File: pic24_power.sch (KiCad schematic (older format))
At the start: 12 parts, among them P2 BAT_CONN, P3 PWR_SWITCH, U1 PIC24EP256GP204, U3 TLV1117

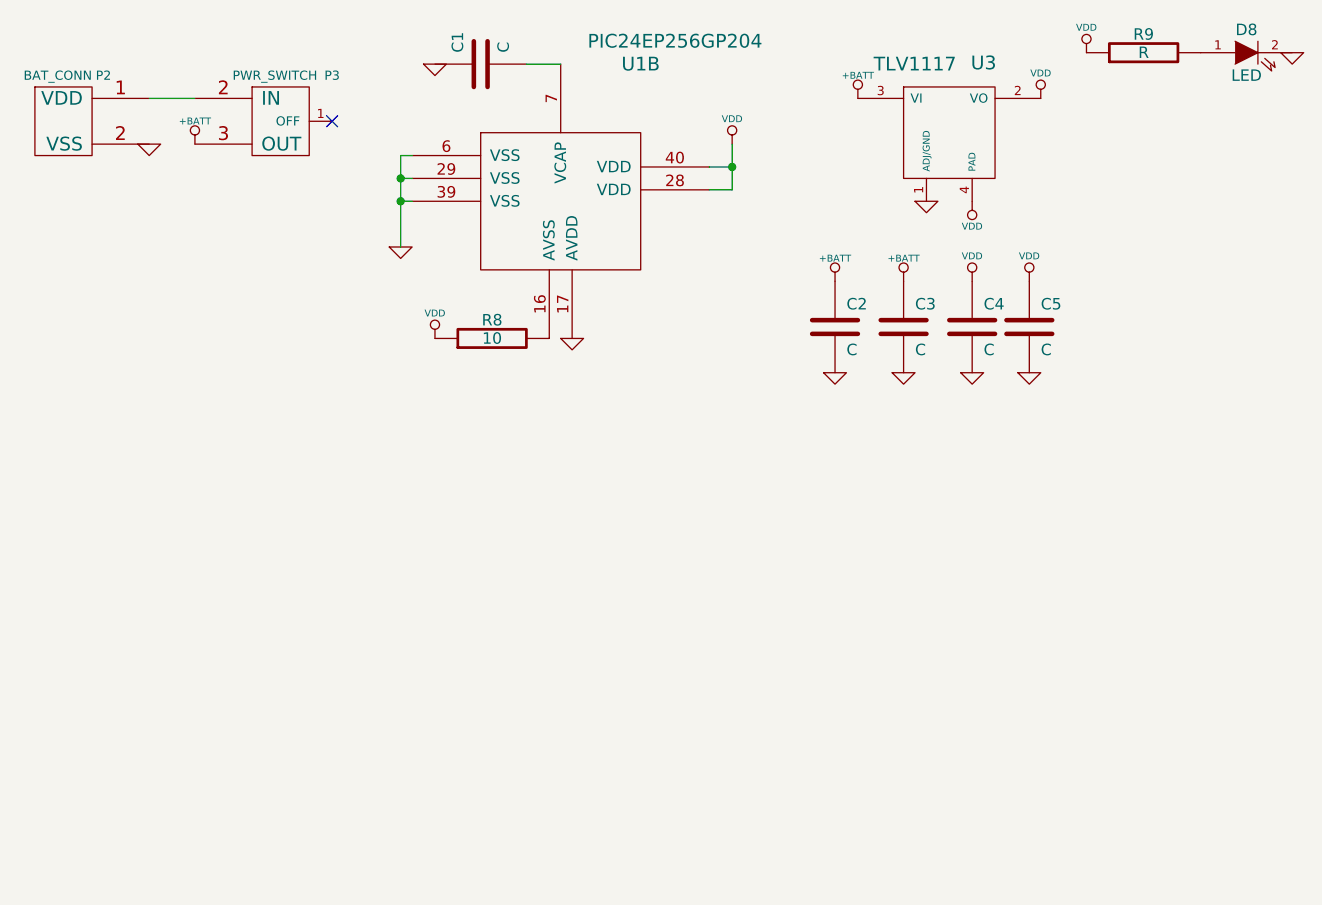
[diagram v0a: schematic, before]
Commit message: checking DFM of the layout
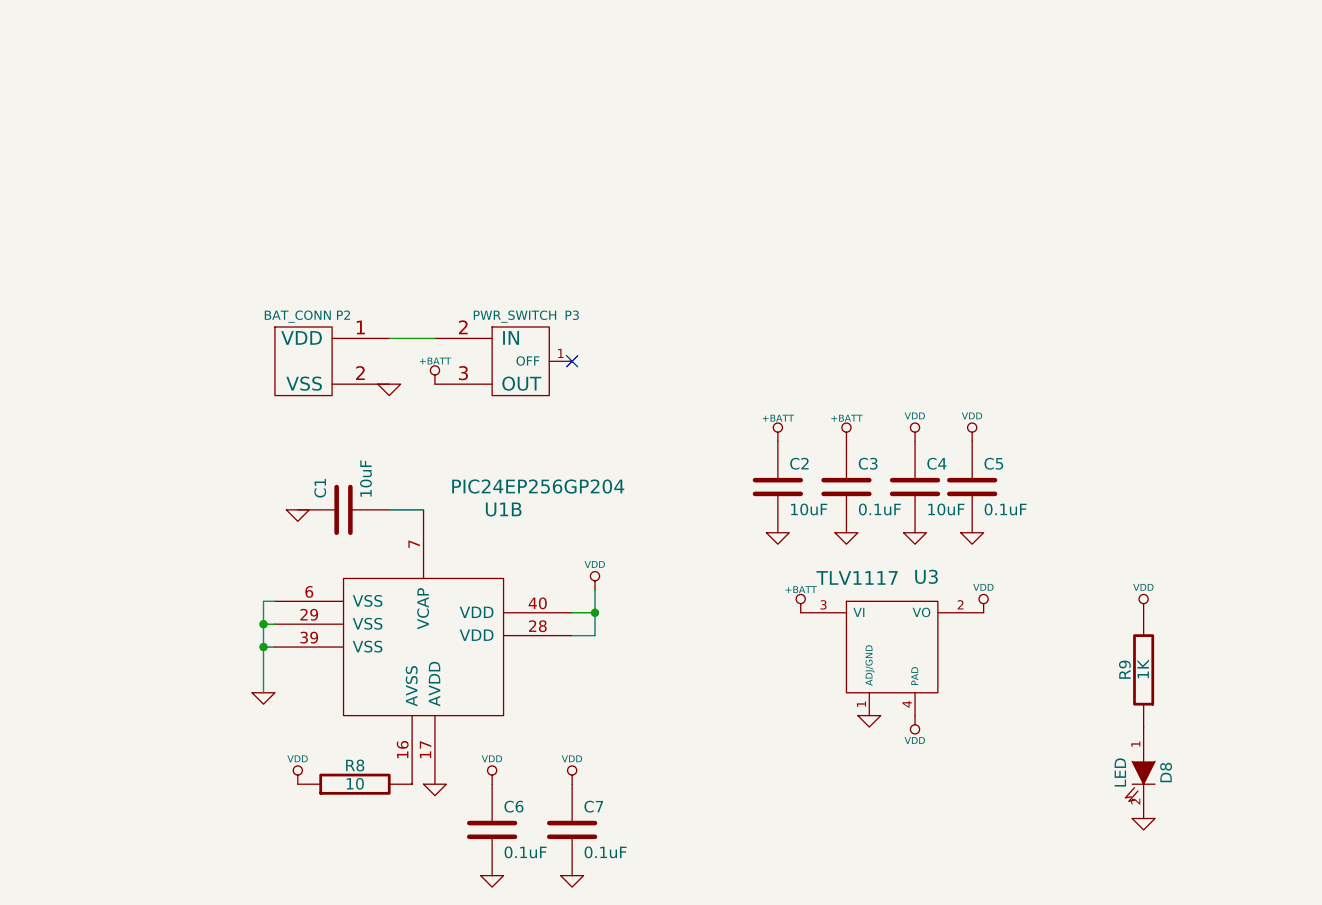
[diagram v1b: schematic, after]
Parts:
- added C6, C7: 0.1uF, symbol C
- C1, C2, C4: value C -> 10uF
- C3, C5: value C -> 0.1uF
- R9: value R -> 1K
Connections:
- net GND: now also C6.2, C7.2
- net VDD: now also R9.2, C6.1, C7.1; no longer R9.1
- net at D8.1 (A): now also R9.1; no longer R9.2
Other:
- moved on the sheet: C1, C2, C3, C4, C5, D8, P2, P3, R8, R9, U1B, U3
